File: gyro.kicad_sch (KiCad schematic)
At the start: 0 parts

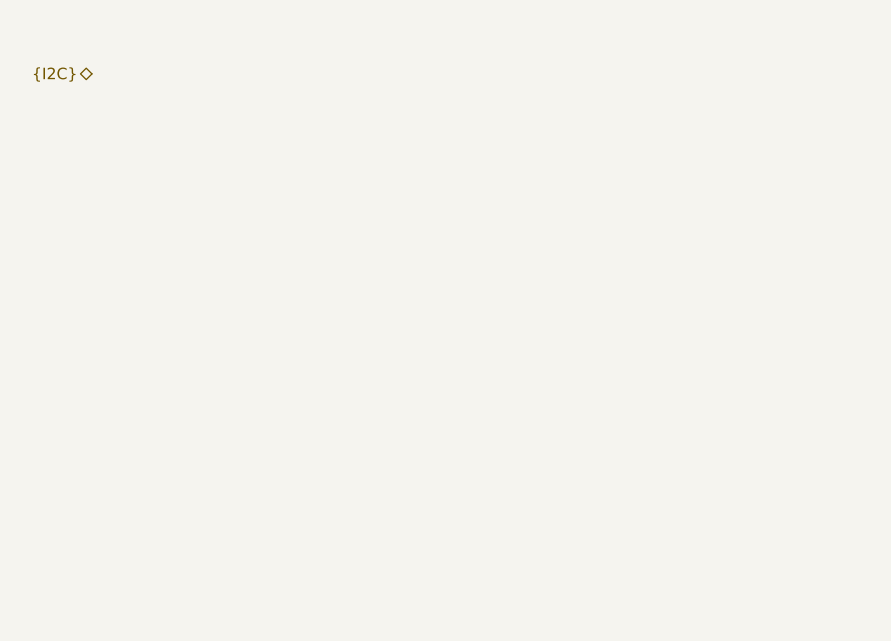
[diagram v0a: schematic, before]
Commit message: Various updates because I forgot to commit for a while
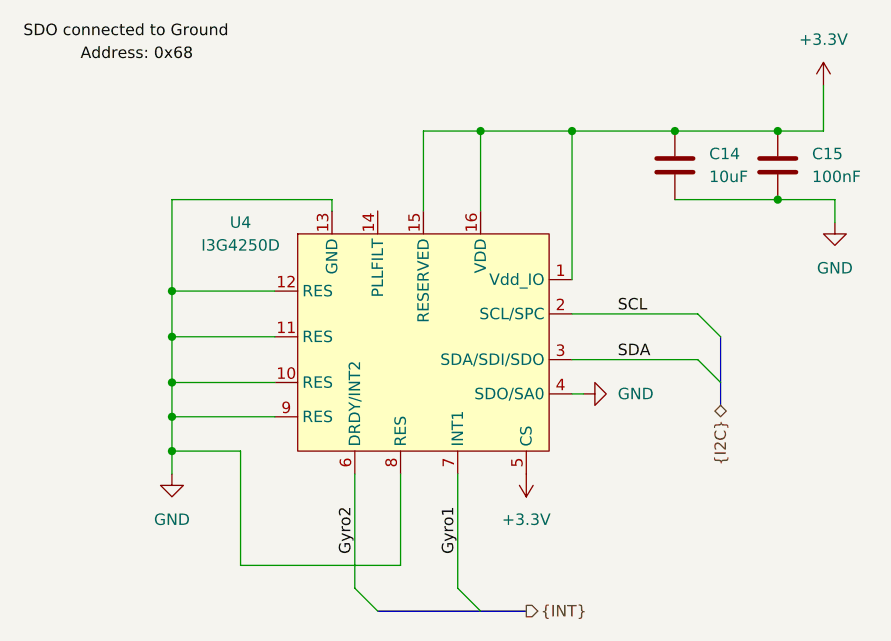
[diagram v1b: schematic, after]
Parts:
- added C14: 10uF, symbol Device:C
- added C15: 100nF, symbol Device:C
- added U4: I3G4250D, symbol Sensor:I3G4250D
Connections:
- new net +3.3V: C14.1, C15.1, U4.1 (Vdd_IO), U4.15 (RESERVED), U4.16 (VDD), U4.5 (CS)
- new net GND: C14.2, C15.2, U4.10 (RES), U4.11 (RES), U4.12 (RES), U4.13 (GND), U4.4 (SDO/SA0), U4.8 (RES), U4.9 (RES)
- new net Gyro1: U4.7 (INT1)
- new net Gyro2: U4.6 (DRDY/INT2)
- new net SCL: U4.2 (SCL/SPC)
- new net SDA: U4.3 (SDA/SDI/SDO)
